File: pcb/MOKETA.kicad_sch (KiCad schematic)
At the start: 85 parts, among them U1 Pro_Micro

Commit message: add footrpint
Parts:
- D1, D10, D11, D12, D13, D14, D15, D16, D17, D18, D19, D2, D20, D21, D22, D23, D24, D25, D26, D27, D28, D29, D3, D30, D31, D32, D33, D34, D35, D36, D37, D38, D39, D4, D40, D41, D42, D5, D6, D7, D8, D9: footprint moketa:D_SOD-323 -> moketa:D_SOD-123
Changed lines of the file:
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@@
 			)
 		)
-		(property "Footprint" "moketa:D_SOD-323"
+		(property "Footprint" "moketa:D_SOD-123"
 			(at 124.968 51.816 0)
 			(effects
@@
 			)
 		)
-		(property "Footprint" "moketa:D_SOD-323"
+		(property "Footprint" "moketa:D_SOD-123"
 			(at 124.968 117.856 0)
 			(effects
@@
 			)
 		)
-		(property "Footprint" "moketa:D_SOD-323"
+		(property "Footprint" "moketa:D_SOD-123"
 			(at 36.068 84.836 0)
 			(effects
@@
 			)
 		)
-		(property "Footprint" "moketa:D_SOD-323"
+		(property "Footprint" "moketa:D_SOD-123"
 			(at 36.068 101.346 0)
 			(effects
@@
 			)
 		)
-		(property "Footprint" "moketa:D_SOD-323"
+		(property "Footprint" "moketa:D_SOD-123"
 			(at 124.968 68.326 0)
 			(effects
@@
 			)
 		)
-		(property "Footprint" "moketa:D_SOD-323"
+		(property "Footprint" "moketa:D_SOD-123"
 			(at 36.068 35.306 0)
 			(effects
@@
 			)
 		)
-		(property "Footprint" "moketa:D_SOD-323"
+		(property "Footprint" "moketa:D_SOD-123"
 			(at 124.968 101.346 0)
 			(effects
@@
 			)
 		)
-		(property "Footprint" "moketa:D_SOD-323"
+		(property "Footprint" "moketa:D_SOD-123"
 			(at 53.848 35.306 0)
 			(effects
@@
 			)
 		)
-		(property "Footprint" "moketa:D_SOD-323"
+		(property "Footprint" "moketa:D_SOD-123"
 			(at 71.628 35.306 0)
 			(effects
@@
 			)
 		)
-		(property "Footprint" "moketa:D_SOD-323"
+		(property "Footprint" "moketa:D_SOD-123"
 			(at 89.408 117.856 0)
 			(effects
@@
 			)
 		)
-		(property "Footprint" "moketa:D_SOD-323"
+		(property "Footprint" "moketa:D_SOD-123"
 			(at 89.408 68.326 0)
 			(effects
@@
 			)
 		)
-		(property "Footprint" "moketa:D_SOD-323"
+		(property "Footprint" "moketa:D_SOD-123"
 			(at 124.968 35.306 0)
 			(effects
@@
 			)
 		)
-		(property "Footprint" "moketa:D_SOD-323"
+		(property "Footprint" "moketa:D_SOD-123"
 			(at 53.848 101.346 0)
 			(effects
@@
 			)
 		)
-		(property "Footprint" "moketa:D_SOD-323"
+		(property "Footprint" "moketa:D_SOD-123"
 			(at 53.848 135.636 0)
 			(effects
@@
 			)
 		)
-		(property "Footprint" "moketa:D_SOD-323"
+		(property "Footprint" "moketa:D_SOD-123"
 			(at 89.408 101.346 0)
 			(effects
@@
 			)
 		)
-		(property "Footprint" "moketa:D_SOD-323"
+		(property "Footprint" "moketa:D_SOD-123"
 			(at 107.188 51.816 0)
 			(effects
@@
 			)
 		)
-		(property "Footprint" "moketa:D_SOD-323"
+		(property "Footprint" "moketa:D_SOD-123"
 			(at 71.628 68.326 0)
 			(effects
@@
 			)
 		)
-		(property "Footprint" "moketa:D_SOD-323"
+		(property "Footprint" "moketa:D_SOD-123"
 			(at 107.188 117.856 0)
 			(effects
@@
 			)
 		)
-		(property "Footprint" "moketa:D_SOD-323"
+		(property "Footprint" "moketa:D_SOD-123"
 			(at 71.628 84.836 0)
 			(effects
@@
 			)
 		)
-		(property "Footprint" "moketa:D_SOD-323"
+		(property "Footprint" "moketa:D_SOD-123"
 			(at 89.408 51.816 0)
 			(effects
@@
 			)
 		)
-		(property "Footprint" "moketa:D_SOD-323"
+		(property "Footprint" "moketa:D_SOD-123"
 			(at 124.968 84.836 0)
 			(effects
@@
 			)
 		)
-		(property "Footprint" "moketa:D_SOD-323"
+		(property "Footprint" "moketa:D_SOD-123"
 			(at 53.848 117.856 0)
 			(effects
@@
 			)
 		)
-		(property "Footprint" "moketa:D_SOD-323"
+		(property "Footprint" "moketa:D_SOD-123"
 			(at 36.068 135.636 0)
 			(effects
@@
 			)
 		)
-		(property "Footprint" "moketa:D_SOD-323"
+		(property "Footprint" "moketa:D_SOD-123"
 			(at 36.068 51.816 0)
 			(effects
@@
 			)
 		)
-		(property "Footprint" "moketa:D_SOD-323"
+		(property "Footprint" "moketa:D_SOD-123"
 			(at 36.068 68.326 0)
 			(effects
@@
 			)
 		)
-		(property "Footprint" "moketa:D_SOD-323"
+		(property "Footprint" "moketa:D_SOD-123"
 			(at 53.848 51.816 0)
 			(effects
@@
 			)
 		)
-		(property "Footprint" "moketa:D_SOD-323"
+		(property "Footprint" "moketa:D_SOD-123"
 			(at 107.188 135.636 0)
 			(effects
@@
 			)
 		)
-		(property "Footprint" "moketa:D_SOD-323"
+		(property "Footprint" "moketa:D_SOD-123"
 			(at 71.628 51.816 0)
 			(effects
@@
 			)
 		)
-		(property "Footprint" "moketa:D_SOD-323"
+		(property "Footprint" "moketa:D_SOD-123"
 			(at 107.188 68.326 0)
 			(effects
@@
 			)
 		)
-		(property "Footprint" "moketa:D_SOD-323"
+		(property "Footprint" "moketa:D_SOD-123"
 			(at 107.188 84.836 0)
 			(effects
@@
 			)
 		)
-		(property "Footprint" "moketa:D_SOD-323"
+		(property "Footprint" "moketa:D_SOD-123"
 			(at 89.408 84.836 0)
 			(effects
@@
 			)
 		)
-		(property "Footprint" "moketa:D_SOD-323"
+		(property "Footprint" "moketa:D_SOD-123"
 			(at 71.628 135.636 0)
 			(effects
@@
 			)
 		)
-		(property "Footprint" "moketa:D_SOD-323"
+		(property "Footprint" "moketa:D_SOD-123"
 			(at 53.848 84.836 0)
 			(effects
@@
 			)
 		)
-		(property "Footprint" "moketa:D_SOD-323"
+		(property "Footprint" "moketa:D_SOD-123"
 			(at 107.188 35.306 0)
 			(effects
@@
 			)
 		)
-		(property "Footprint" "moketa:D_SOD-323"
+		(property "Footprint" "moketa:D_SOD-123"
 			(at 107.188 101.346 0)
 			(effects
@@
 			)
 		)
-		(property "Footprint" "moketa:D_SOD-323"
+		(property "Footprint" "moketa:D_SOD-123"
 			(at 124.968 135.636 0)
 			(effects
@@
 			)
 		)
-		(property "Footprint" "moketa:D_SOD-323"
+		(property "Footprint" "moketa:D_SOD-123"
 			(at 36.068 117.856 0)
 			(effects
@@
 			)
 		)
-		(property "Footprint" "moketa:D_SOD-323"
+		(property "Footprint" "moketa:D_SOD-123"
 			(at 71.628 117.856 0)
 			(effects
@@
 			)
 		)
-		(property "Footprint" "moketa:D_SOD-323"
+		(property "Footprint" "moketa:D_SOD-123"
 			(at 71.628 101.346 0)
 			(effects
@@
 			)
 		)
-		(property "Footprint" "moketa:D_SOD-323"
+		(property "Footprint" "moketa:D_SOD-123"
 			(at 53.848 68.326 0)
 			(effects
@@
 			)
 		)
-		(property "Footprint" "moketa:D_SOD-323"
+		(property "Footprint" "moketa:D_SOD-123"
 			(at 89.408 35.306 0)
 			(effects
@@
 			)
 		)
-		(property "Footprint" "moketa:D_SOD-323"
+		(property "Footprint" "moketa:D_SOD-123"
 			(at 89.408 135.636 0)
 			(effects

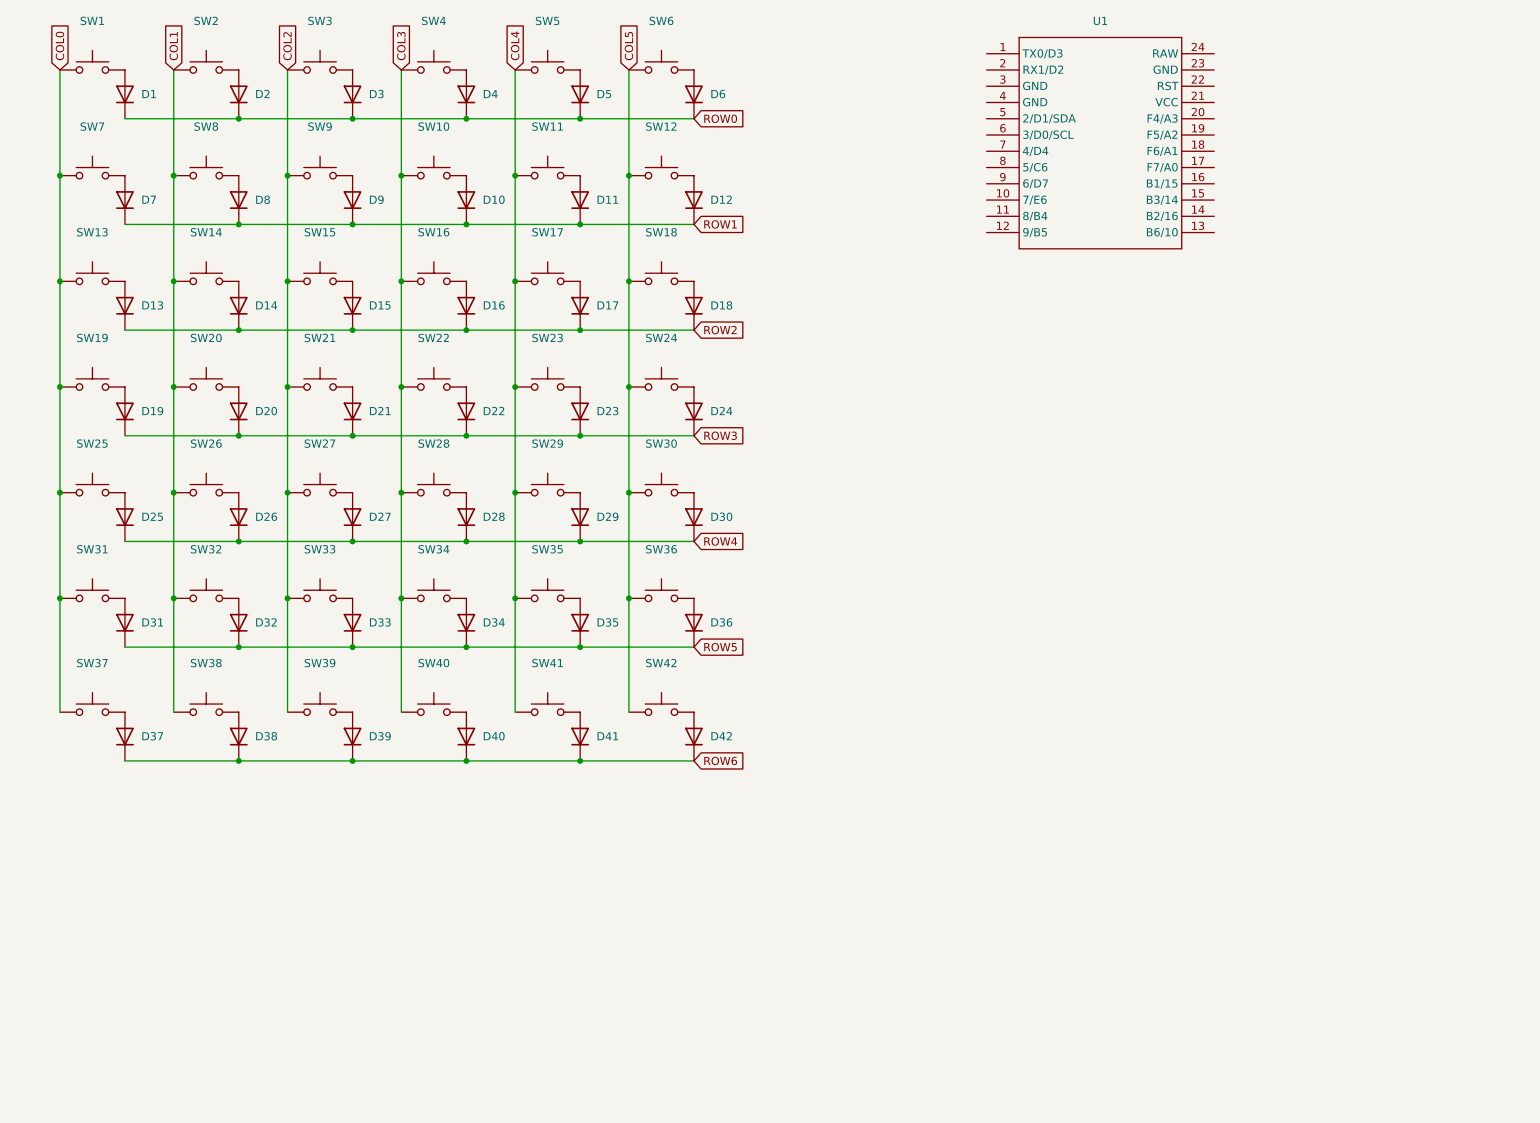
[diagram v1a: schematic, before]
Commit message: update footprint
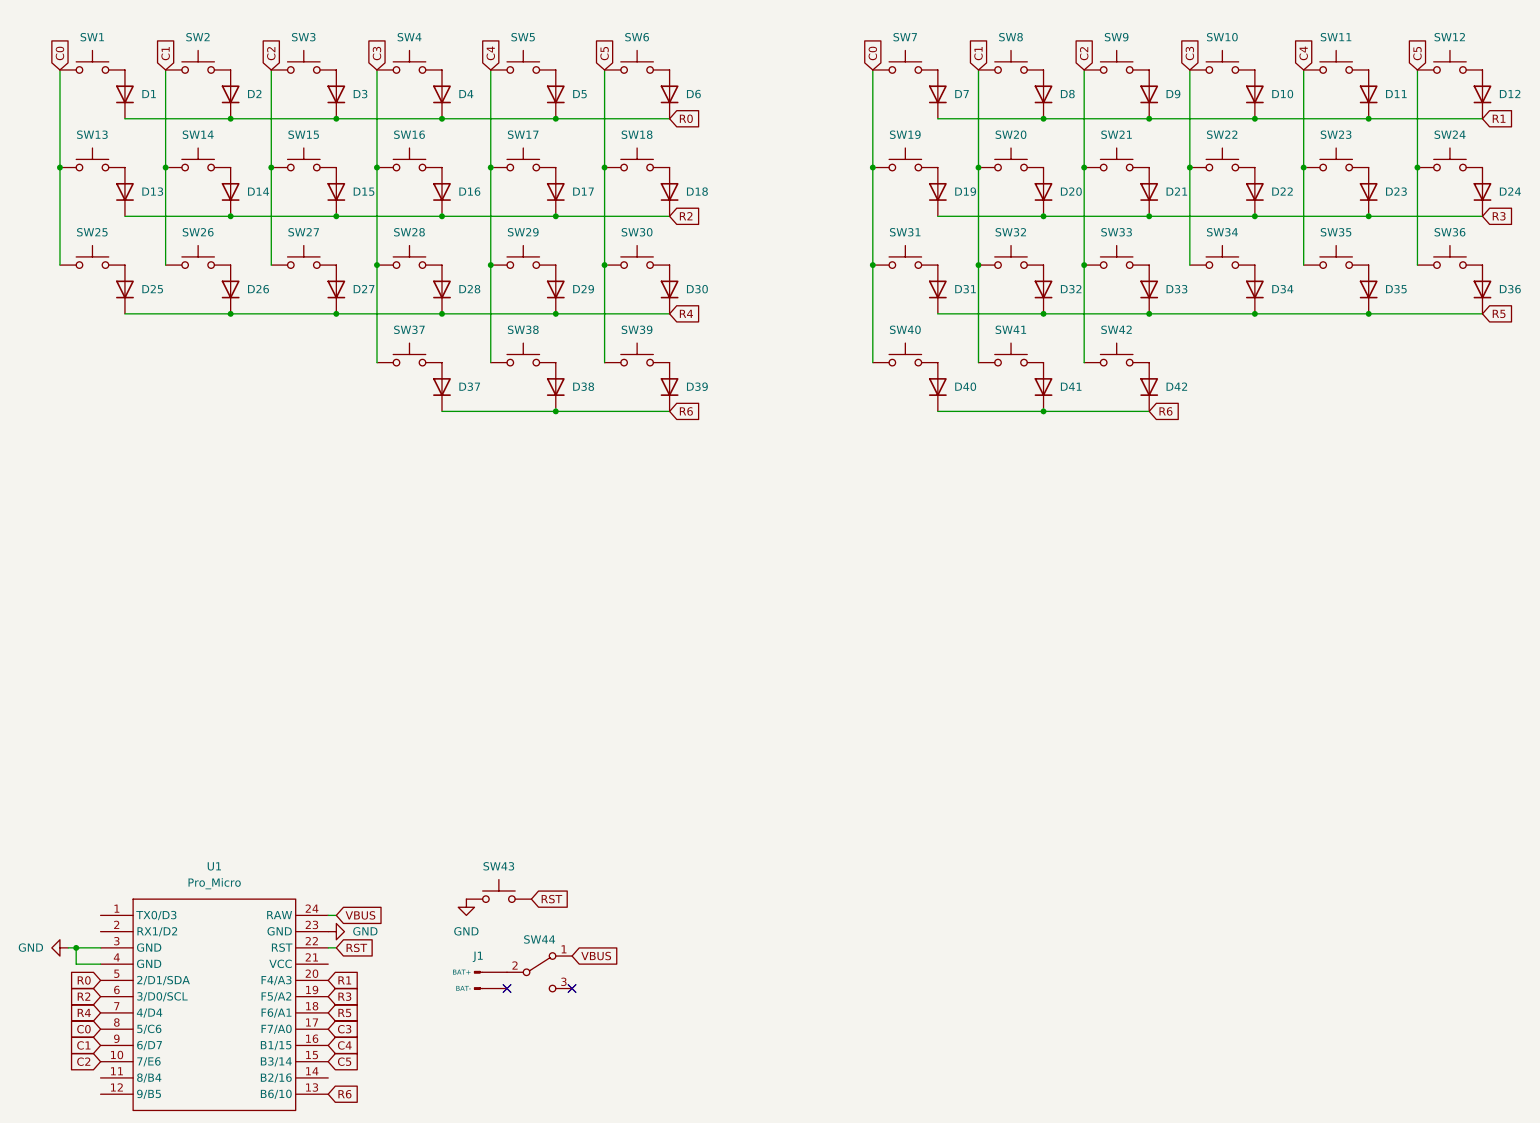
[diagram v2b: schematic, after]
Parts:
- removed SW1, SW10, SW11, SW12, SW13, SW14, SW15, SW16, SW17, SW18, SW19, SW2, SW20, SW21, SW22, SW23, SW24, SW25, SW26, SW27, SW28, SW29, SW3, SW30, SW31, SW32, SW33, SW34, SW35, SW36, SW37, SW38, SW39, SW4, SW40, SW41, SW42, SW5, SW6, SW7, SW8, SW9: ~, moketa:SW_PUSH, symbol moketa:Tact_Switch
- added J1: ~, symbol moketa:J_BATTERY
- added SW1, SW10, SW11, SW12, SW13, SW14, SW15, SW16, SW17, SW18, SW19, SW2, SW20, SW21, SW22, SW23, SW24, SW25, SW26, SW27, SW28, SW29, SW3, SW30, SW31, SW32, SW33, SW34, SW35, SW36, SW37, SW38, SW39, SW4, SW40, SW41, SW42, SW5, SW6, SW7, SW8, SW9: ~, moketa:SW_PUSH, symbol moketa:SW_PUSH
- added SW43: Reset, symbol moketa:SW_TACT
- added SW44: ~, symbol moketa:SW_SLIDE
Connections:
- net ROW0 is gone; now on net R0: D1.1 (K), D2.1 (K), D3.1 (K), D4.1 (K), D5.1 (K), D6.1 (K)
- net ROW1 is gone; now on net R1: D10.1 (K), D11.1 (K), D12.1 (K), D7.1 (K), D8.1 (K), D9.1 (K)
- net ROW2 is gone; now on net R2: D13.1 (K), D14.1 (K), D15.1 (K), D16.1 (K), D17.1 (K), D18.1 (K)
- net ROW3 is gone; now on net R3: D19.1 (K), D20.1 (K), D21.1 (K), D22.1 (K), D23.1 (K), D24.1 (K)
- net ROW4 is gone; now on net R4: D25.1 (K), D26.1 (K), D27.1 (K), D28.1 (K), D29.1 (K), D30.1 (K)
- net ROW5 is gone; now on net R5: D31.1 (K), D32.1 (K), D33.1 (K), D34.1 (K), D35.1 (K), D36.1 (K)
- net ROW6 is gone; now on net R6: D37.1 (K), D38.1 (K), D39.1 (K), D40.1 (K), D41.1 (K), D42.1 (K)
- net at D30.2 (A): now also SW30.2
- net at D6.2 (A): now also SW6.2
- net at D12.2 (A): now also SW12.2
- net at D36.2 (A): now also SW36.2
- net at D32.2 (A): now also SW32.2
- net at D19.2 (A): now also SW19.2
- net C2: now reaches U1.10 (7/E6)
- net C2: now also SW15.1, SW21.1, SW27.1, SW3.1, SW33.1, SW42.1, SW9.1
- net R6: now reaches U1.13 (B6/10)
- net C5: now reaches U1.15 (B3/14)
- net C5: now also SW12.1, SW18.1, SW24.1, SW30.1, SW36.1, SW39.1, SW6.1
- net C4: now reaches U1.16 (B1/15)
- net C4: now also SW11.1, SW17.1, SW23.1, SW29.1, SW35.1, SW38.1, SW5.1
- net C3: now reaches U1.17 (F7/A0)
- net C3: now also SW10.1, SW16.1, SW22.1, SW28.1, SW34.1, SW37.1, SW4.1
- net R5: now reaches U1.18 (F6/A1)
- net R3: now reaches U1.19 (F5/A2)
- net R1: now reaches U1.20 (F4/A3)
- net RST: now reaches U1.22 (RST)
- net RST: now also SW43.2
- net GND: now reaches U1.23 (GND)
- net GND: now also U1.3 (GND), U1.4 (GND), SW43.1
- net VBUS: now reaches U1.24 (RAW)
- net VBUS: now also SW44.1 (A)
- net R0: now reaches U1.5 (2/D1/SDA)
- net R2: now reaches U1.6 (3/D0/SCL)
- net R4: now reaches U1.7 (4/D4)
- net C0: now reaches U1.8 (5/C6)
- net C0: now also SW1.1, SW13.1, SW19.1, SW25.1, SW31.1, SW40.1, SW7.1
- net C1: now reaches U1.9 (6/D7)
- net C1: now also SW14.1, SW2.1, SW20.1, SW26.1, SW32.1, SW41.1, SW8.1
- net at D23.2 (A): now also SW23.2
- net at D2.2 (A): now also SW2.2
- net at D7.2 (A): now also SW7.2
- net at D25.2 (A): now also SW25.2
- net at D11.2 (A): now also SW11.2
- net at D34.2 (A): now also SW34.2
- net at D3.2 (A): now also SW3.2
- net at D9.2 (A): now also SW9.2
- net at D40.2 (A): now also SW40.2
- net at D10.2 (A): now also SW10.2
- net at D39.2 (A): now also SW39.2
- net at D15.2 (A): now also SW15.2
- net at D18.2 (A): now also SW18.2
- net at D24.2 (A): now also SW24.2
- net at D1.2 (A): now also SW1.2
- net at D41.2 (A): now also SW41.2
- net at D20.2 (A): now also SW20.2
- net at D16.2 (A): now also SW16.2
- net at D26.2 (A): now also SW26.2
- net at D38.2 (A): now also SW38.2
- net at D28.2 (A): now also SW28.2
- net at D22.2 (A): now also SW22.2
- net at D35.2 (A): now also SW35.2
- net at D17.2 (A): now also SW17.2
- net at D31.2 (A): now also SW31.2
- net at D21.2 (A): now also SW21.2
- net at D8.2 (A): now also SW8.2
- net at D4.2 (A): now also SW4.2
- net at D29.2 (A): now also SW29.2
- net at D27.2 (A): now also SW27.2
- net at D37.2 (A): now also SW37.2
- net at D13.2 (A): now also SW13.2
- net at D5.2 (A): now also SW5.2
- net at D42.2 (A): now also SW42.2
- net at D14.2 (A): now also SW14.2
- net at D33.2 (A): now also SW33.2
- new net: J1.1 (BAT+), SW44.2 (B)
- no-connect marks 0 -> 2
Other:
- moved on the sheet: U1
